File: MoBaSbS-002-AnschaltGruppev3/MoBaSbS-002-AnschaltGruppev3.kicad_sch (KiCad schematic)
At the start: 28 parts, among them J1 RJ45, J2 RJ45, J3 Conn_02x04_Top_Bottom, J4 Conn_02x04_Top_Bottom, P1 PSS254, P4 2x5_Buchse, P5 Wago, P6 Wago

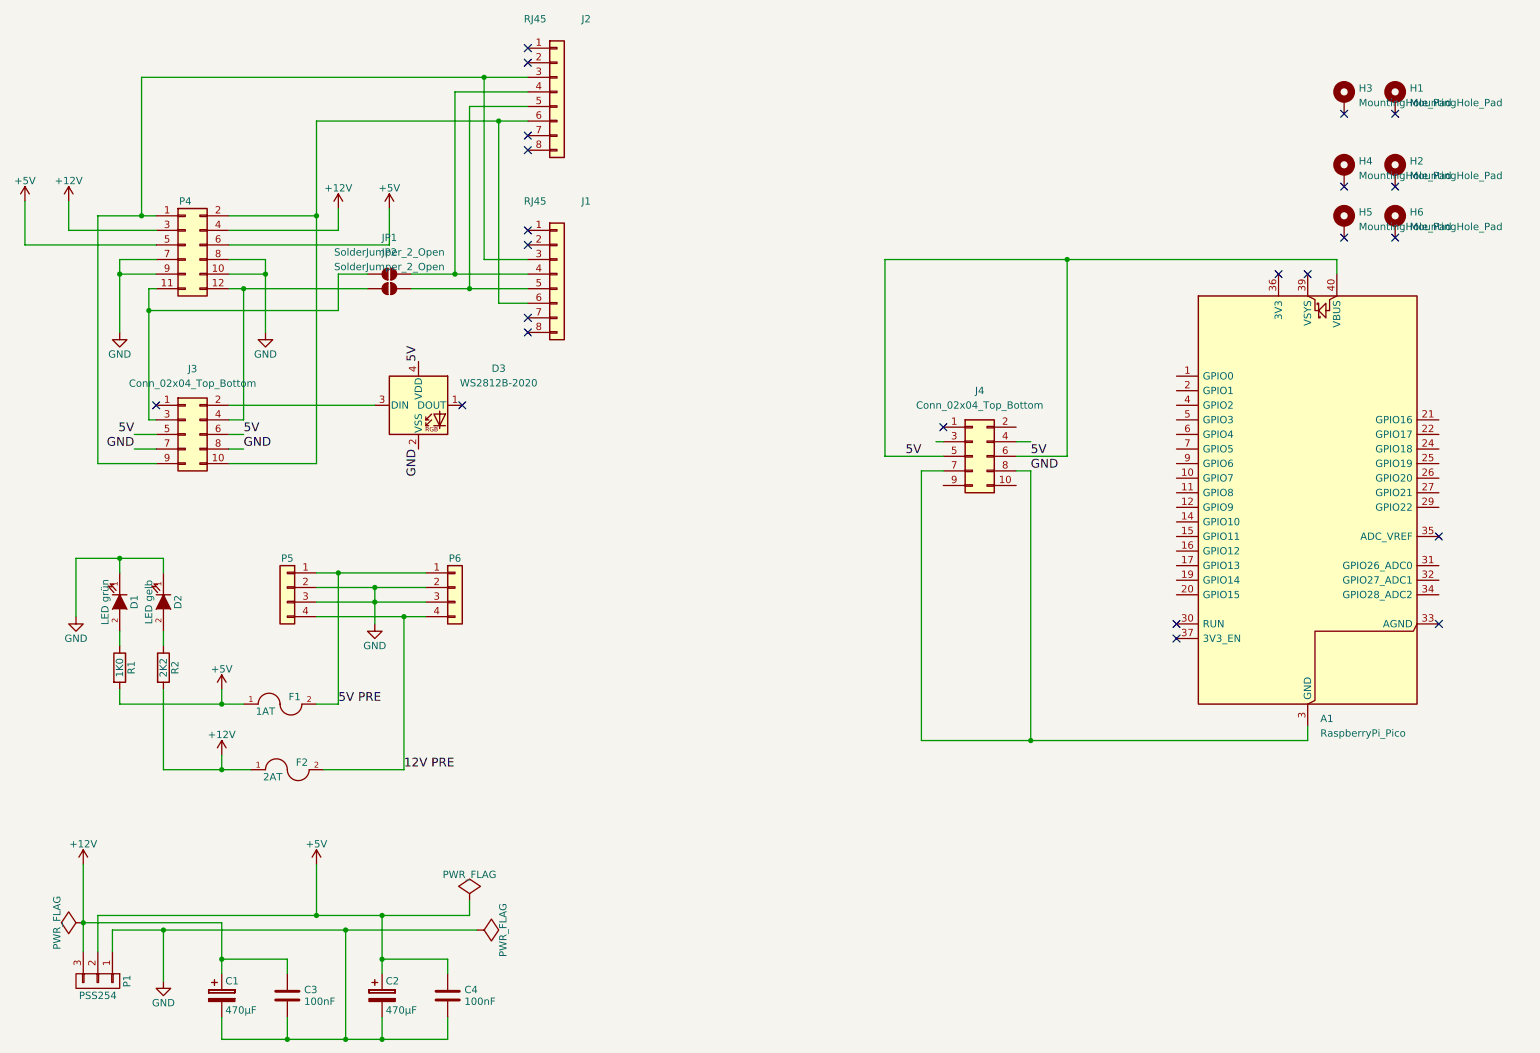
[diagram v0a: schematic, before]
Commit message: More work on the PCB
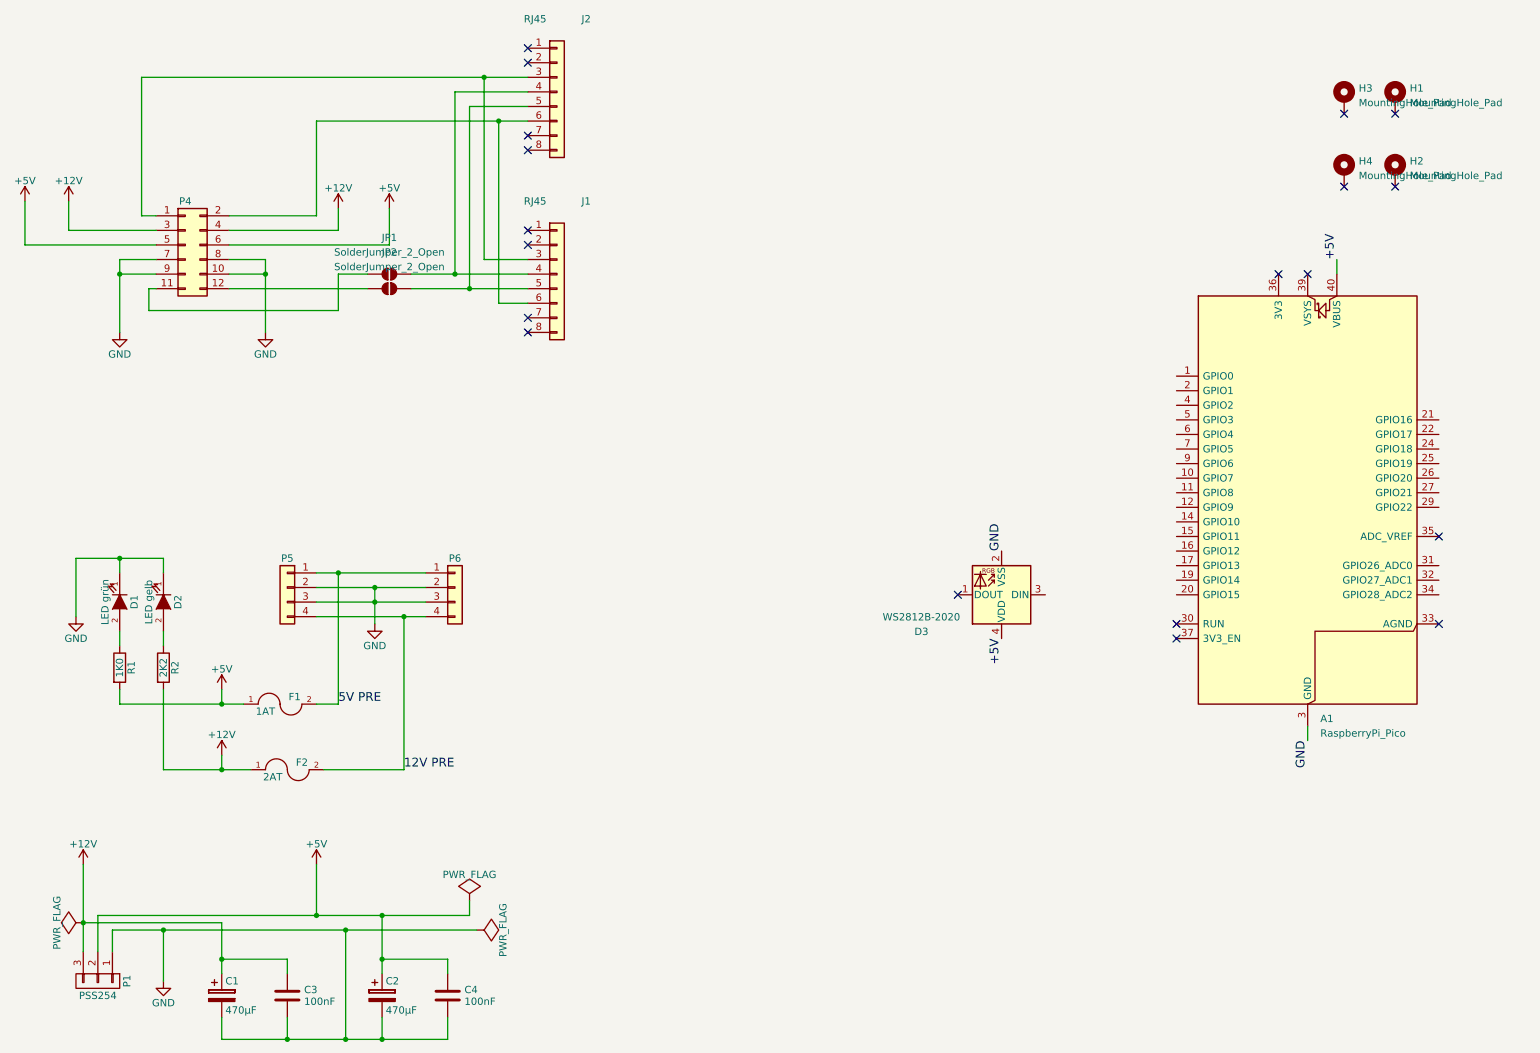
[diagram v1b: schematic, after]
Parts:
- removed H5, H6: MountingHole_Pad, MountingHole:MountingHole_2.7mm_M2.5_DIN965_Pad, symbol Mechanical:MountingHole_Pad
- removed J3: Conn_02x04_Top_Bottom, Connector_PinSocket_2.54mm:PinSocket_2x05_P2.54mm_Horizontal, symbol Connector_Generic:Conn_02x05_Odd_Even
- removed J4: Conn_02x04_Top_Bottom, Connector_PinHeader_2.54mm:PinHeader_2x05_P2.54mm_Horizontal, symbol Connector_Generic:Conn_02x05_Odd_Even
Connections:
- net 5V is gone; now on net +5V: A1.40 (VBUS), D3.4 (VDD)
- no-connect marks 23 -> 19
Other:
- moved on the sheet: D3
